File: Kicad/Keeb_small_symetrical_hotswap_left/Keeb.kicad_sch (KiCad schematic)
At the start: 32 parts, among them J1 TYPE-C-31-M-12, J2 B2B-XH-A_LF__SN_, SW1 CherryMX, SW10 CherryMX, SW11 CherryMX, SW13 CherryMX, SW14 CherryMX, SW15 CherryMX, SW16 CherryMX, SW17 CherryMX, SW18 CherryMX, SW19 CherryMX, SW2 CherryMX, SW20 CherryMX, SW3 CherryMX, SW4 CherryMX, SW5 CherryMX, SW6 CherryMX, SW7 CherryMX, SW8 CherryMX, SW9 CherryMX, U1 Pico, U2 KY-040

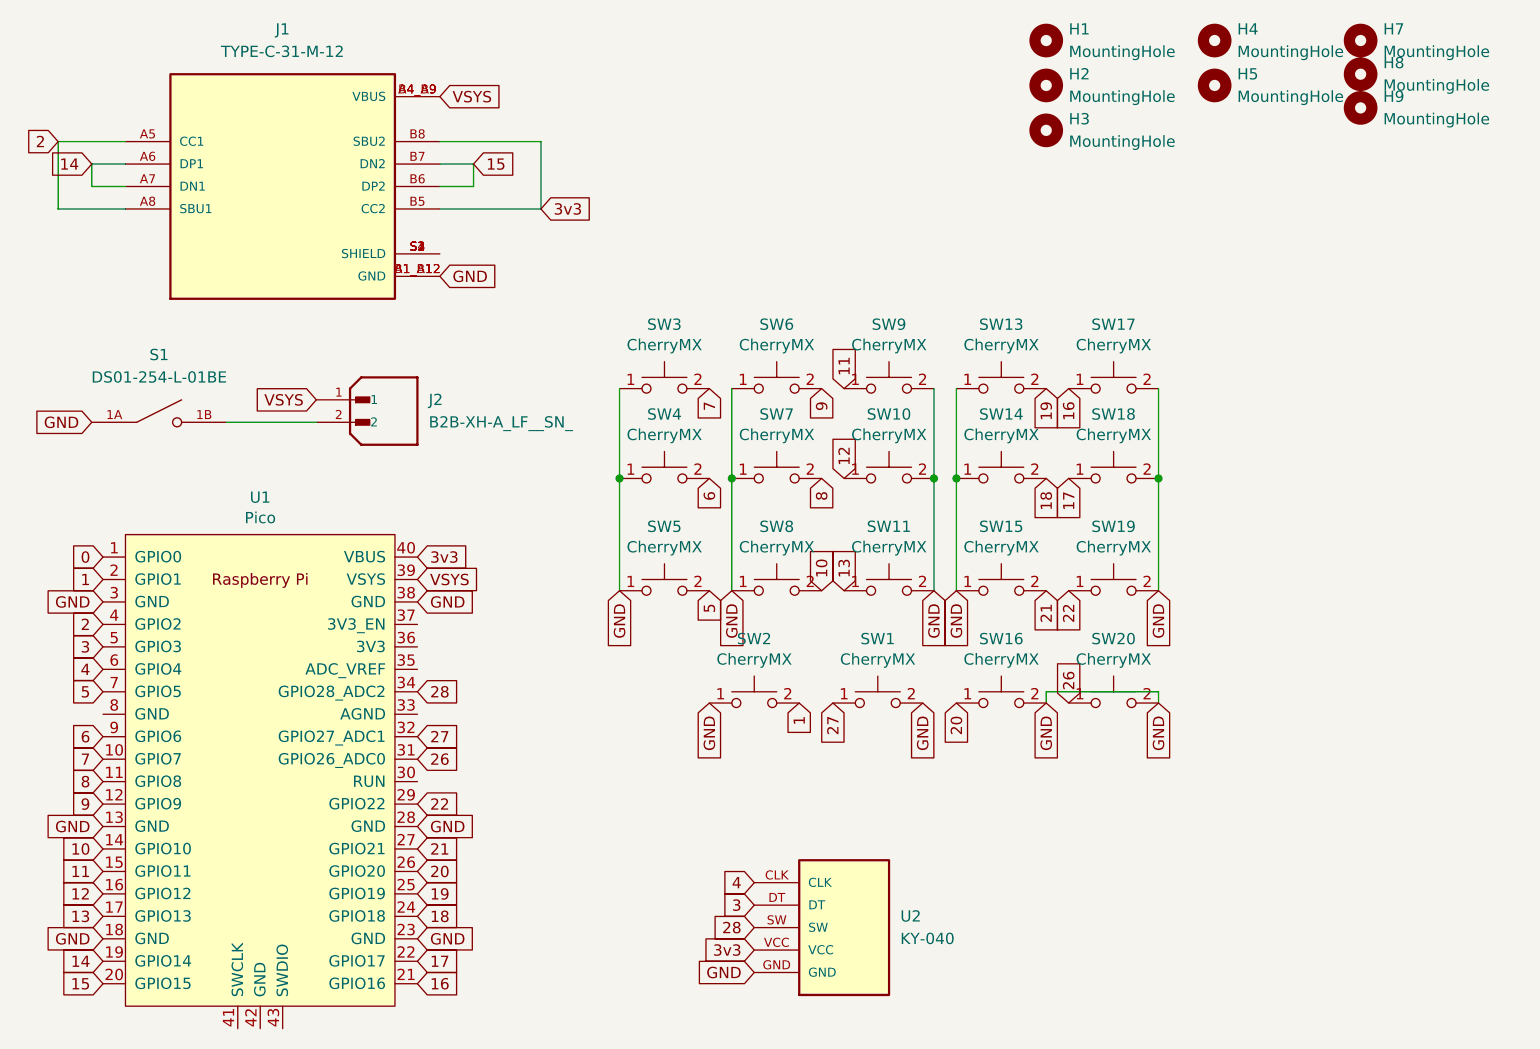
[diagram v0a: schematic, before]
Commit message: Initial commit
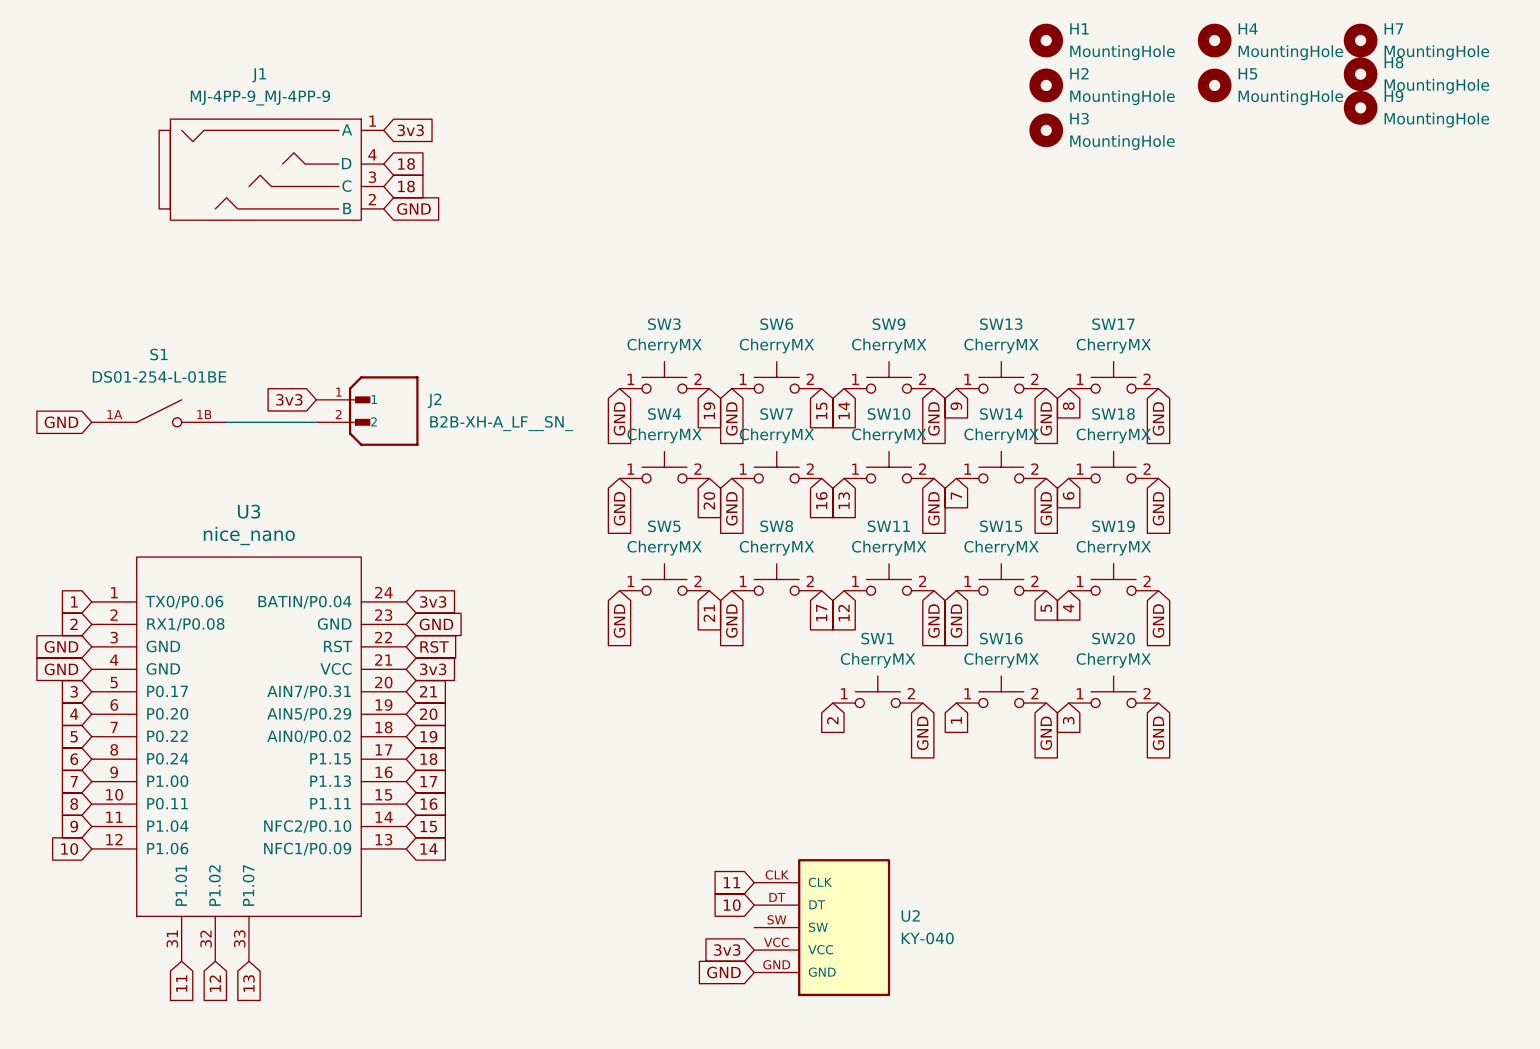
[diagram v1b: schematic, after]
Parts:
- removed J1: TYPE-C-31-M-12, TypeC:HRO_TYPE-C-31-M-12, symbol TypeC:TYPE-C-31-M-12
- removed SW2: CherryMX, ScottoKeebs_Hotswap:Hotswap_MX_Plated_1.00u_Smaller_hole, symbol Keeb-rescue:CherryMX-CherryMX
- removed U1: Pico, MCU_RaspberryPi_and_Boards:RPi_Pico_SMD_TH_NO_BACK_HOLES, symbol Keeb-rescue:Pico-MCU_RaspberryPi_and_Boards
- added J1: MJ-4PP-9_MJ-4PP-9, MJ-4PP-9:MJ-4PP-9, symbol Keeb-rescue:MJ-4PP-9-MJ-4PP-9
- added U3: nice_nano, Nice_nano:nice_nano, symbol nice_nano:nice_nano
- SW1, SW10, SW11, SW13, SW14, SW15, SW16, SW17, SW18, SW19, SW20, SW3, SW4, SW5, SW6, SW7, SW8, SW9: footprint ScottoKeebs_Hotswap:Hotswap_MX_Plated_1.00u_Smaller_hole -> ScottoKeebs_Hotswap:Hotswap_MX_Plated_1.00u
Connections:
- net 22 is gone; now on net 4: SW19.1
- net 26 is gone; now on net 3: SW20.1
- net 27 is gone; now on net 2: SW1.1
- net VSYS is gone; now on net 3v3: J2.1
- net 1: now also SW16.1, U3.1 (TX0/P0.06)
- net 10: now also U2.DT, U3.12 (P1.06); no longer SW8.2
- net 11: now also U2.CLK, U3.31 (P1.01); no longer SW9.1
- net 12: now also SW11.1, U3.32 (P1.02); no longer SW10.1
- net 13: now also SW10.1, U3.33 (P1.07); no longer SW11.1
- net 14: now also SW9.1, U3.13 (NFC1/P0.09)
- net 15: now also SW6.2, U3.14 (NFC2/P0.10)
- net 16: now also SW7.2, U3.15 (P1.11); no longer SW17.1
- net 17: now also SW8.2, U3.16 (P1.13); no longer SW18.1
- net 18: now also J1.3 (C), J1.4 (D), U3.17 (P1.15); no longer SW14.2
- net 19: now also SW3.2, U3.18 (AIN0/P0.02); no longer SW13.2
- net 2: now also U3.2 (RX1/P0.08)
- net 20: now also SW4.2, U3.19 (AIN5/P0.29); no longer SW16.1
- net 21: now also SW5.2, U3.20 (AIN7/P0.31); no longer SW15.2
- net 3: now also U3.5 (P0.17); no longer U2.DT
- net 3v3: now also J1.1 (A), U3.21 (VCC), U3.24 (BATIN/P0.04)
- net 4: now also U3.6 (P0.20); no longer U2.CLK
- net 5: now also SW15.2, U3.7 (P0.22); no longer SW5.2
- net 6: now also SW18.1, U3.8 (P0.24); no longer SW4.2
- net 7: now also SW14.1, U3.9 (P1.00); no longer SW3.2
- net 8: now also SW17.1, U3.10 (P0.11); no longer SW7.2
- net 9: now also SW13.1, U3.11 (P1.04); no longer SW6.2
- net GND: now also SW13.2, SW14.2, J1.2 (B), U3.23 (GND), U3.3 (GND), U3.4 (GND); no longer SW13.1, SW14.1
- net 28: no longer names the net of U2.SW
- new net RST: U3.22 (RST)
